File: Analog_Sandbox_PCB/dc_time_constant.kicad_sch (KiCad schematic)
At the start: 1 part

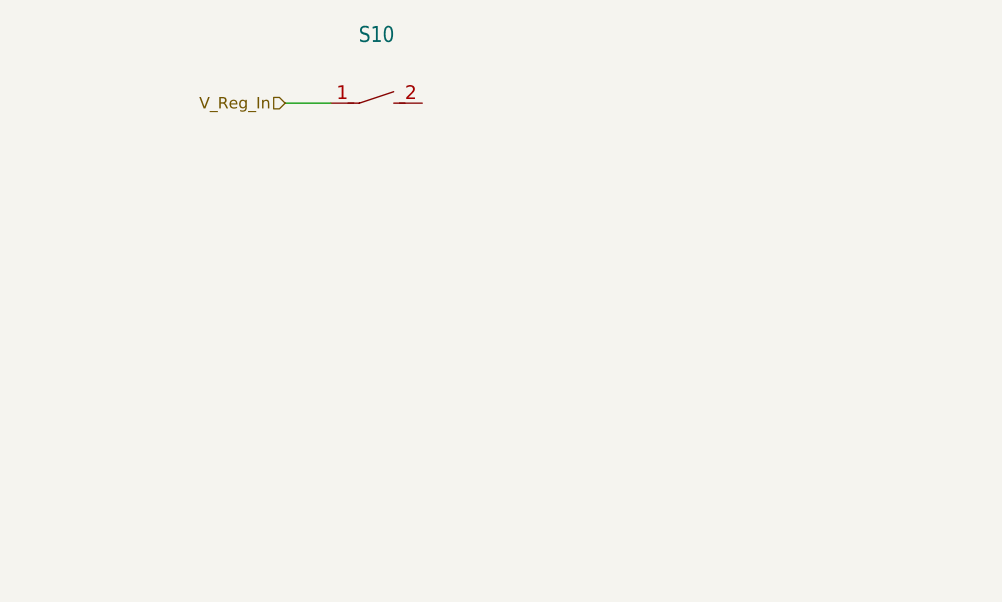
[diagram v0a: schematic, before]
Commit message: All Circuits Added, Layout Almost done
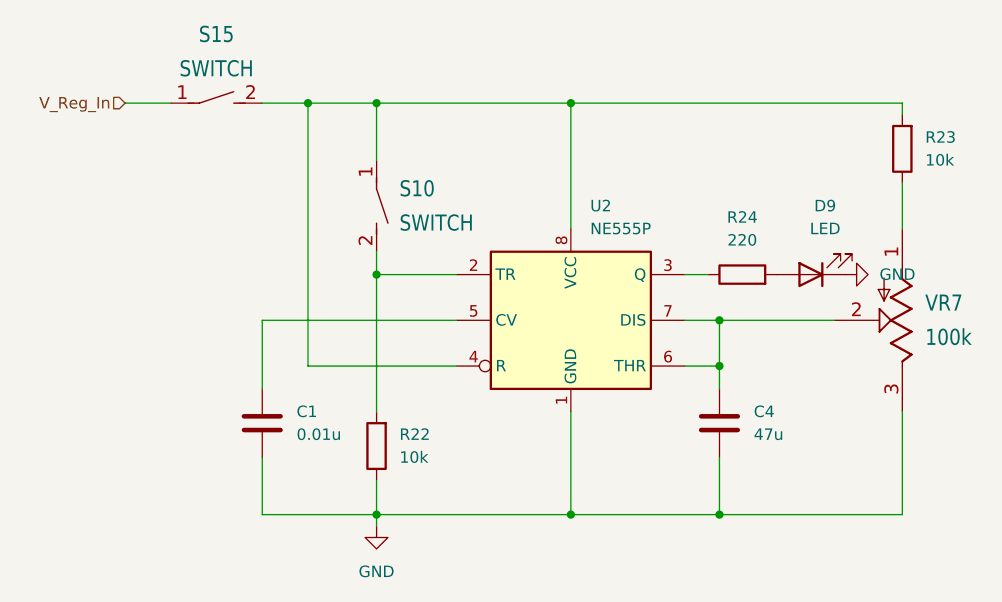
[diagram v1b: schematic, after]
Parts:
- added C1: 0.01u, symbol Device:C
- added C4: 47u, symbol Device:C
- added D9: LED, Diode_SMD:D_1206_3216Metric, symbol Device:LED
- added R22, R23: 10k, Resistor_SMD:R_2010_5025Metric_Pad1.40x2.65mm_HandSolder, symbol Device:R
- added R24: 220, Resistor_SMD:R_2010_5025Metric_Pad1.40x2.65mm_HandSolder, symbol Device:R
- added S15: SWITCH, Button_Switch_THT:SW_DIP_SPSTx01_Slide_9.78x4.72mm_W7.62mm_P2.54mm, symbol Analog_Sandbox_PCB-eagle-import:DS01E
- added U2: NE555P, Package_DIP:DIP-8_W7.62mm, symbol Timer:NE555P
- added VR7: 100k, Analog_Sandbox_PCB:TRIM_3362P-1-102LF, symbol Analog_Sandbox_PCB-eagle-import:3362P-1-102LF
- S10: value ~ -> SWITCH; footprint Analog_Sandbox_PCB:DS-01 -> Button_Switch_THT:SW_DIP_SPSTx01_Slide_9.78x4.72mm_W7.62mm_P2.54mm
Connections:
- net V_Reg_In: now also S15.1; no longer S10.1
- net at S10.2: now also R22.2, U2.2 (TR)
- new net: R23.2, S10.1, S15.2, U2.4 (R), U2.8 (VCC)
- new net: C4.1, U2.6 (THR), U2.7 (DIS), VR7.2 (WIPER)
- new net: R23.1, VR7.1 (CCW)
- new net: C1.1, U2.5 (CV)
- new net: D9.2 (A), R24.2
- new net: R24.1, U2.3 (Q)
- new net GND: C1.2, C4.2, D9.1 (K), R22.1, U2.1 (GND), VR7.3 (CW)
